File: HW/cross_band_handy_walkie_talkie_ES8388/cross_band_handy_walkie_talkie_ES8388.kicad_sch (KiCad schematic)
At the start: 108 parts, among them J1 USB_C_Receptacle, J10 Conn_01x04, J2 Micro_SD_Card_Det, J9 Conn_01x04, Q1 nMOS, Q2 AO3401A, Q3 AO3401A, Q4 AO3401A, Q6 nMOS, SW1 MCU_RESET, SW2 MCU_RESET, U1 SRV05-4, U2 ESP32-S3-WROOM-1, U3 AMS1117-3.3, U4 TP5000

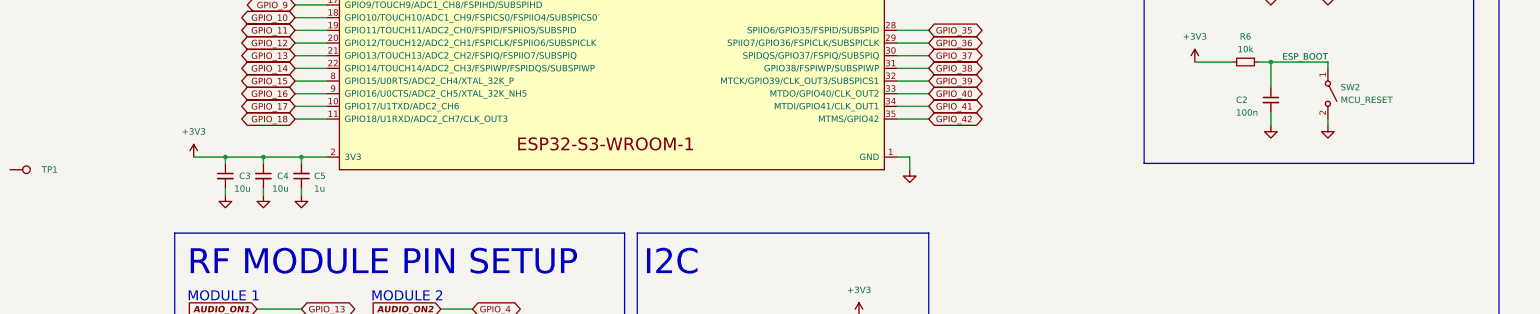
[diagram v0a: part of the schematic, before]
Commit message: f
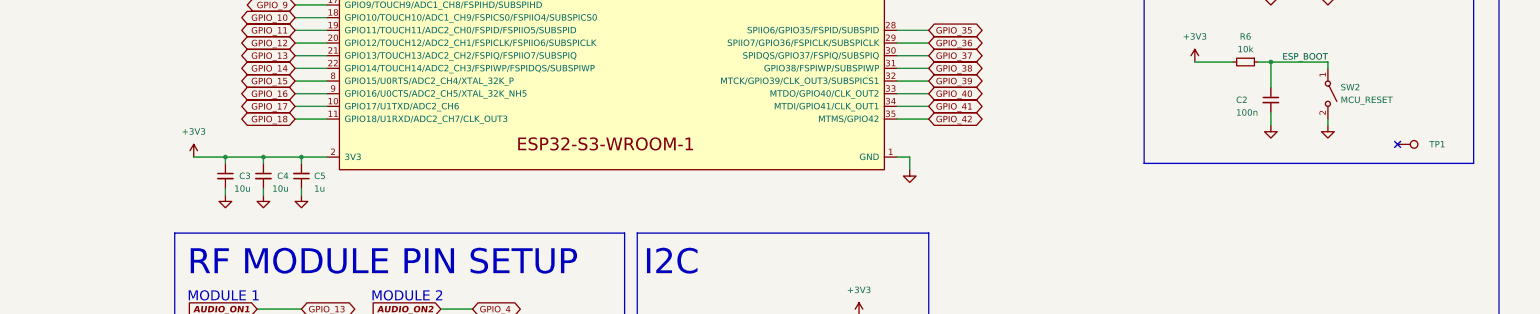
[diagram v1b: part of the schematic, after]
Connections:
- no-connect marks 16 -> 17
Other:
- moved on the sheet: TP1
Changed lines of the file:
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@@
   (no_connect (at 355.6 71.12))
   (no_connect (at 247.65 265.43))
+  (no_connect (at 260.35 93.98))
   (no_connect (at 355.6 78.74))
   (no_connect (at 355.6 93.98))
@@
     (pin "1")
   )
-  (symbol (lib_id "Connector:TestPoint") (at -17.78 99.06 270) (unit 1)
+  (symbol (lib_id "Connector:TestPoint") (at 260.35 93.98 270) (unit 1)
     (in_bom no) (on_board no) (fields_autoplaced)
-    (property "Reference" "TP1" (id 0) (at -11.43 99.0599 90)
+    (property "Reference" "TP1" (id 0) (at 266.7 93.9799 90)
       (effects (font (size 1.27 1.27)) (justify left))
     )
-    (property "Value" "TestPoint" (id 1) (at -15.7479 102.87 0)
+    (property "Value" "TestPoint" (id 1) (at 262.3821 97.79 0)
       (effects (font (size 1.27 1.27)) (justify left) hide)
     )
-    (property "Footprint" "TestPoint:TestPoint_Pad_1.0x1.0mm" (id 2) (at -17.78 104.14 0)
+    (property "Footprint" "TestPoint:TestPoint_Pad_1.0x1.0mm" (id 2) (at 260.35 99.06 0)
       (effects (font (size 1.27 1.27)) hide)
     )
-    (property "Datasheet" "~" (id 3) (at -17.78 104.14 0)
+    (property "Datasheet" "~" (id 3) (at 260.35 99.06 0)
       (effects (font (size 1.27 1.27)) hide)
     )
